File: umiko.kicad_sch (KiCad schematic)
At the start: 398 parts, among them J1 USB_C_Receptacle_USB2.0, J2 USB_C_Receptacle_USB2.0, J3 USB_C_Receptacle_USB2.0, J4 USB_C_Receptacle_USB2.0, SW1 SWITCH, SW2 SWITCH, U1 USBLC6-2P6, U10 TLV75533PDQNR, U11 RP2040, U2 TLV75533PDQNR, U3 W25Q128JVPIQ, U5 SN74LVC1T45DRL, U6 W25Q128JVPIQ, U7 RP2040, U8 SN74LVC1T45DRL, U9 USBLC6-2P6, Y1 12MHz, Y2 12MHz

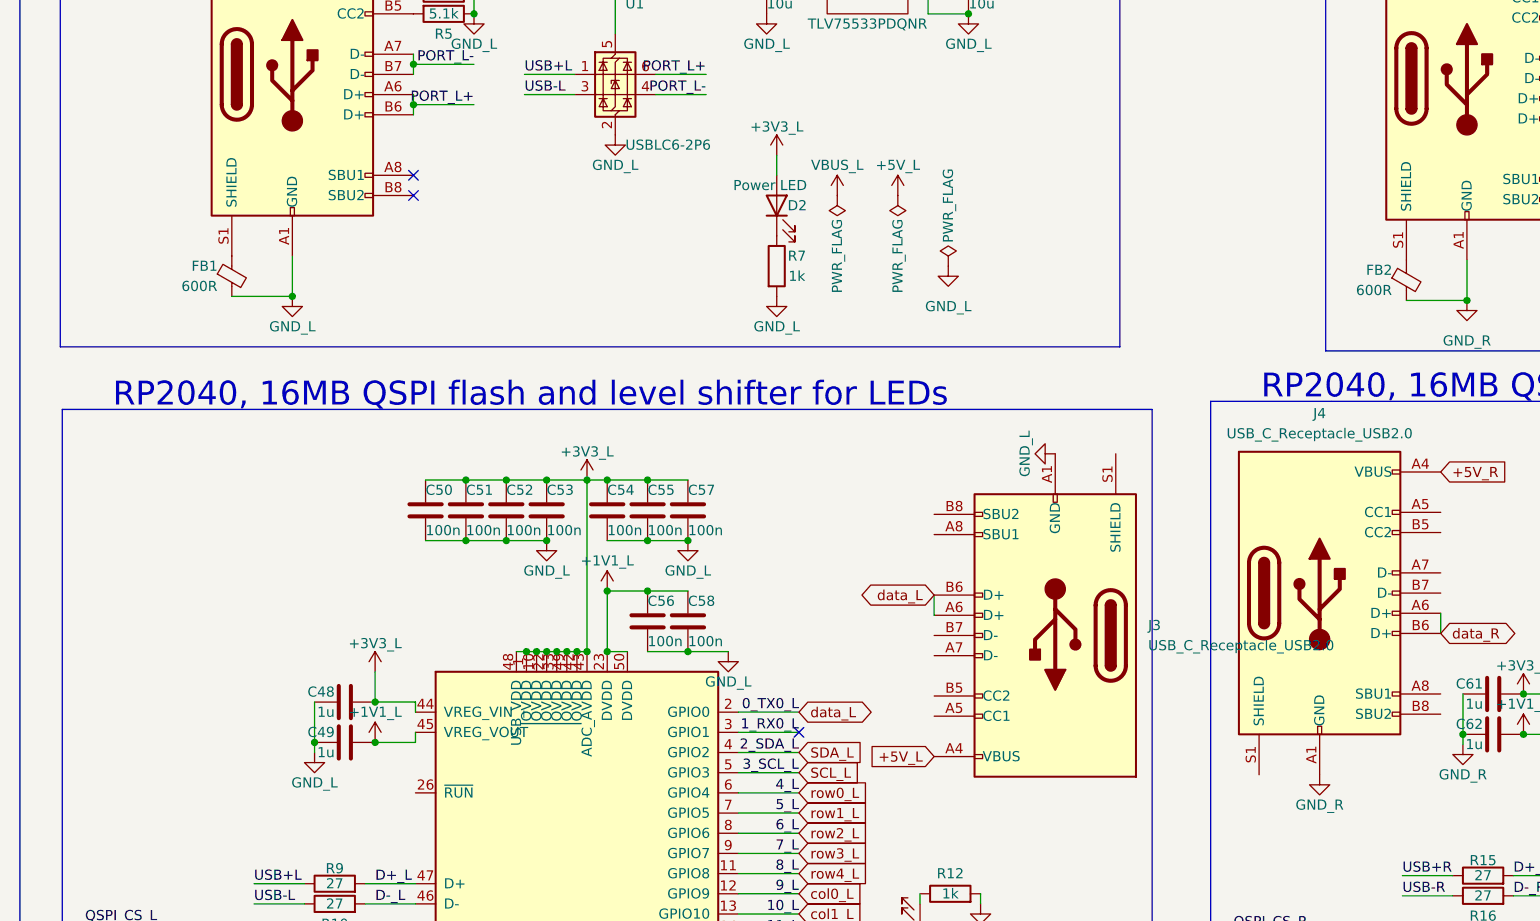
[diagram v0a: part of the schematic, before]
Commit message: USB-C shield: expose S2/S3/S4 in symbol + J2 area routing pass
Schematic: added S2/S3/S4 SHIELD pins to the embedded
Connector:USB_C_Receptacle_USB2.0 symbol so all four shield/mounting pads
can be wired (previously only S1 was exposed). PCB: routing pass on the
right host USB-C (J2) area.

Co-Authored-By: Claude Opus 4.7 <noreply@anthropic.com>
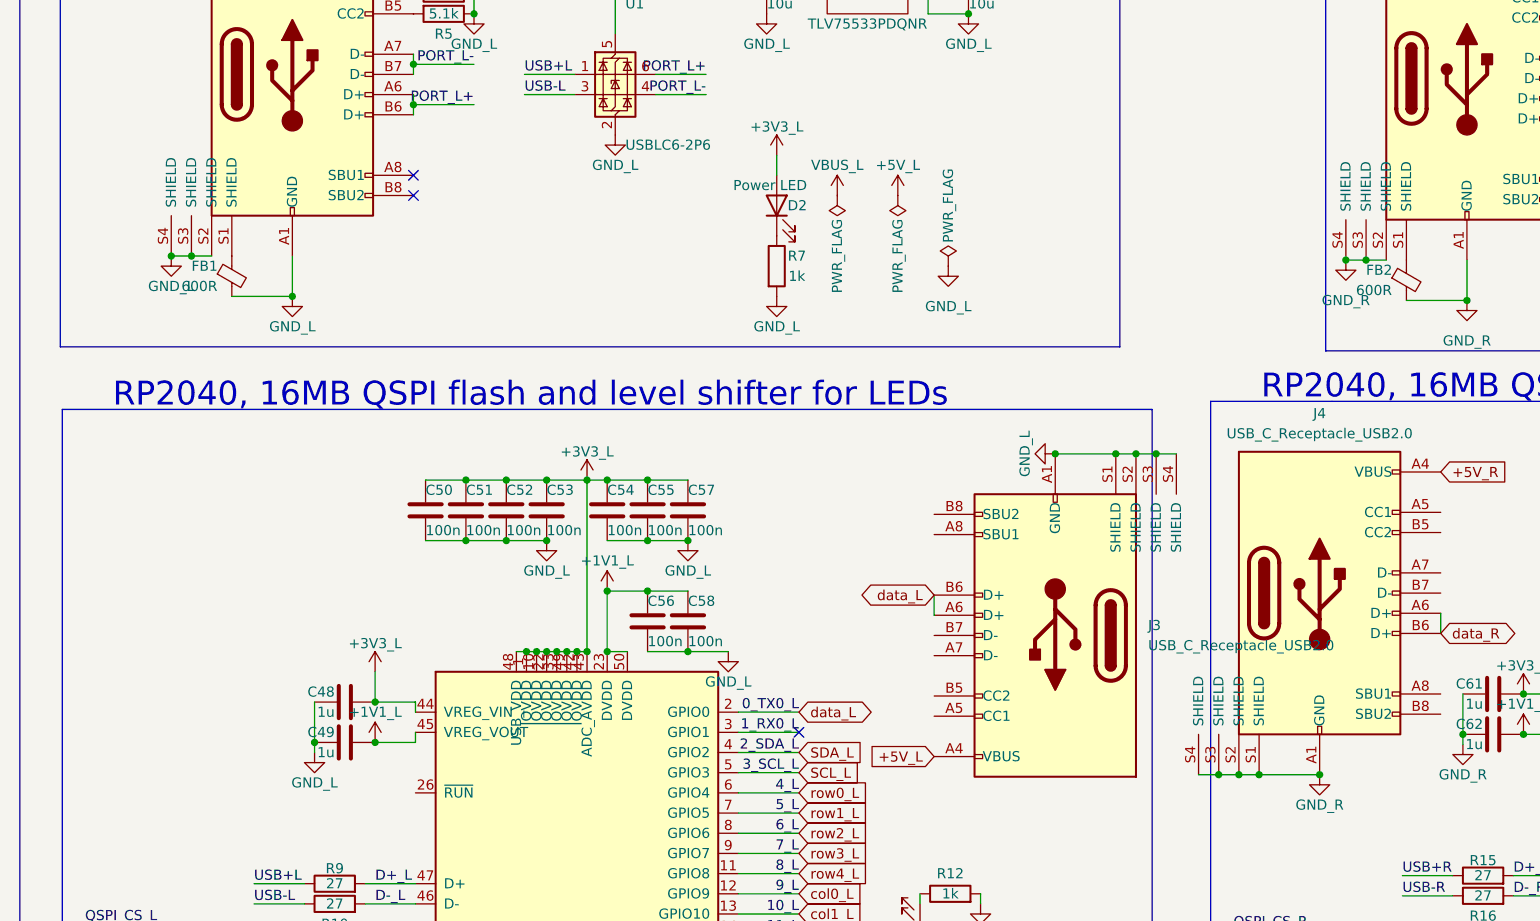
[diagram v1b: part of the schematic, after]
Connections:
- net GND_L: now also J1.S2 (SHIELD), J1.S3 (SHIELD), J1.S4 (SHIELD), J3.S1 (SHIELD), J3.S2 (SHIELD), J3.S3 (SHIELD), J3.S4 (SHIELD)
- net GND_R: now also J2.S2 (SHIELD), J2.S3 (SHIELD), J2.S4 (SHIELD), J4.S1 (SHIELD), J4.S2 (SHIELD), J4.S3 (SHIELD), J4.S4 (SHIELD)
